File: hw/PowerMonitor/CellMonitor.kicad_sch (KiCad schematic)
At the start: 25 parts, among them Q1 Q_PMOS_GDS, U5 LM358, U6 LM358, U7 LM358, U8 LM393, U9 74LVC1G32

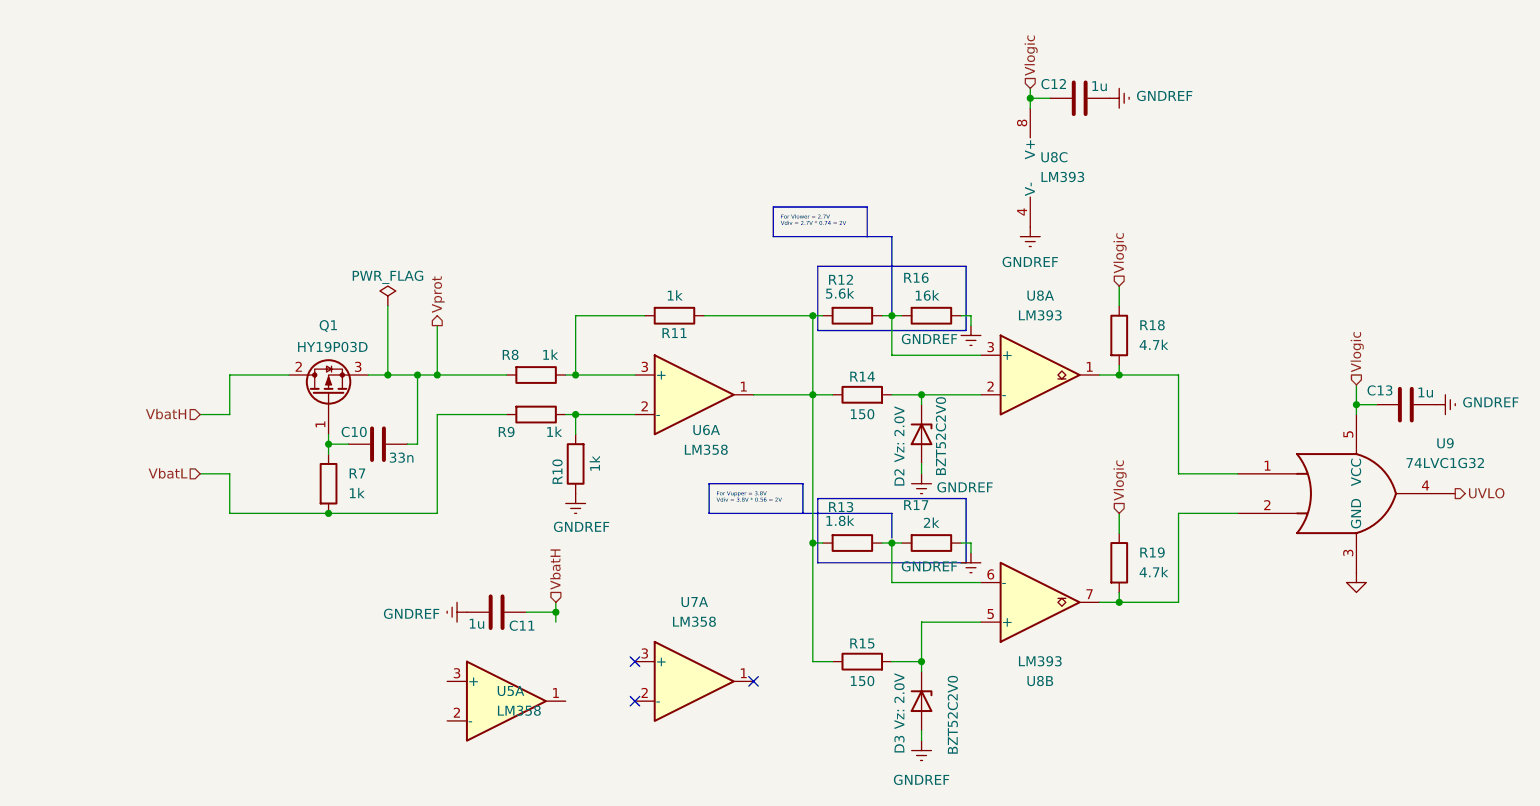
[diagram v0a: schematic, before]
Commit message: Rework powermon
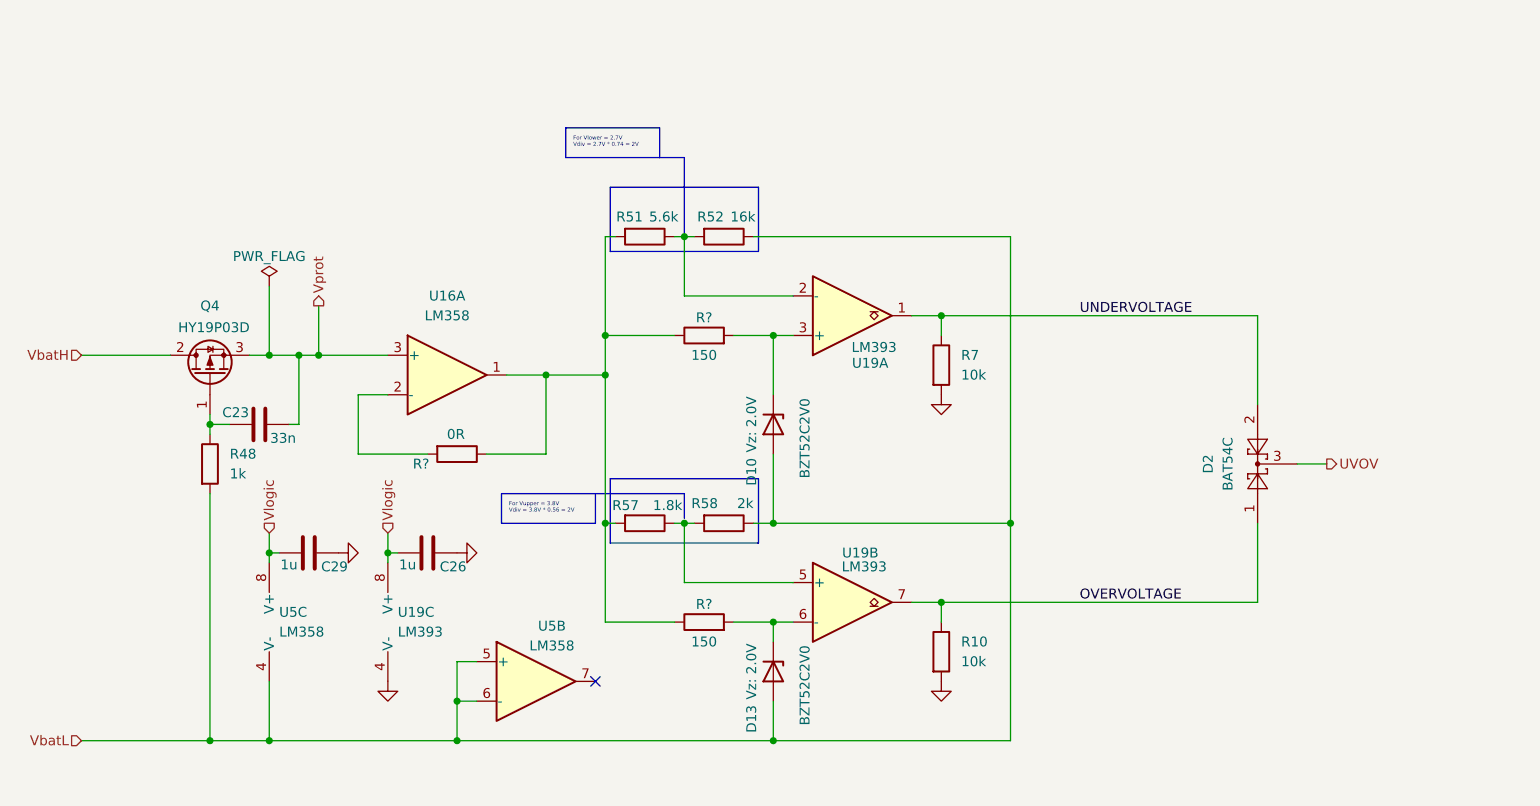
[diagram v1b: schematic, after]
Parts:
- removed C10: 33n, Capacitor_SMD:C_0603_1608Metric_Pad1.08x0.95mm_HandSolder, symbol Device:C
- removed C11, C12, C13: 1u, Capacitor_SMD:C_0603_1608Metric_Pad1.08x0.95mm_HandSolder, symbol Device:C
- removed D2, D3: BZT52Bxx, Diode_SMD:D_SOD-123F, symbol Diode:BZT52Bxx
- removed Q1: Q_PMOS_GDS, Package_TO_SOT_SMD:TO-252-2, symbol Transistor_FET:Q_PMOS_GDS
- removed R11, R8, R9: 1k, Resistor_SMD:R_0603_1608Metric_Pad0.98x0.95mm_HandSolder, symbol Device:R
- removed R12: 5.6k, Resistor_SMD:R_0603_1608Metric_Pad0.98x0.95mm_HandSolder, symbol Device:R
- removed R13: 1.8k, Resistor_SMD:R_0603_1608Metric_Pad0.98x0.95mm_HandSolder, symbol Device:R
- removed R14, R15: 150, Resistor_SMD:R_0603_1608Metric_Pad0.98x0.95mm_HandSolder, symbol Device:R
- removed R16: 16k, Resistor_SMD:R_0603_1608Metric_Pad0.98x0.95mm_HandSolder, symbol Device:R
- removed R17: 2k, Resistor_SMD:R_0603_1608Metric_Pad0.98x0.95mm_HandSolder, symbol Device:R
- removed R18, R19: 4.7k, Resistor_SMD:R_0603_1608Metric_Pad0.98x0.95mm_HandSolder, symbol Device:R
- removed U5, U6, U7: LM358, Package_SO:SOIC-8_3.9x4.9mm_P1.27mm, symbol Amplifier_Operational:LM358
- removed U8: LM393, Package_SO:SOIC-8_3.9x4.9mm_P1.27mm, symbol Comparator:LM393
- removed U9: 74LVC1G32, Package_TO_SOT_SMD:SOT-353_SC-70-5_Handsoldering, symbol 74xGxx:74LVC1G32
- added C23: 33n, Capacitor_SMD:C_0603_1608Metric_Pad1.08x0.95mm_HandSolder, symbol Device:C
- added C26, C29: 1u, Capacitor_SMD:C_0603_1608Metric_Pad1.08x0.95mm_HandSolder, symbol Device:C
- added D10, D13: BZT52Bxx, Diode_SMD:D_SOD-123F, symbol Diode:BZT52Bxx
- added D2: BAT54C, Package_TO_SOT_SMD:SOT-23_Handsoldering, symbol Diode:BAT54C
- added Q4: Q_PMOS_GDS, Package_TO_SOT_SMD:TO-252-2, symbol Transistor_FET:Q_PMOS_GDS
- added R48: 1k, Resistor_SMD:R_0603_1608Metric_Pad0.98x0.95mm_HandSolder, symbol Device:R
- added R51: 5.6k, Resistor_SMD:R_0603_1608Metric_Pad0.98x0.95mm_HandSolder, symbol Device:R
- added R52: 16k, Resistor_SMD:R_0603_1608Metric_Pad0.98x0.95mm_HandSolder, symbol Device:R
- added R57: 1.8k, Resistor_SMD:R_0603_1608Metric_Pad0.98x0.95mm_HandSolder, symbol Device:R
- added R58: 2k, Resistor_SMD:R_0603_1608Metric_Pad0.98x0.95mm_HandSolder, symbol Device:R
- added R?: 0R, Resistor_SMD:R_0603_1608Metric_Pad0.98x0.95mm_HandSolder, symbol Device:R
- added R? (x2): 150, Resistor_SMD:R_0603_1608Metric_Pad0.98x0.95mm_HandSolder, symbol Device:R
- added U16, U5: LM358, Package_SO:SOIC-8_3.9x4.9mm_P1.27mm, symbol Amplifier_Operational:LM358
- added U19: LM393, Package_SO:SOIC-8_3.9x4.9mm_P1.27mm, symbol Comparator:LM393
- R10, R7: value 1k -> 10k
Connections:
- net GND: now also R10.2, R7.2, C26.1, C29.1, U19.4 (V-)
- net VbatH: now also Q4.2 (D)
- net VbatL: now also D10.2 (A), D13.2 (A), R48.2, R52.1, R58.1, U5.4 (V-), U5.5 (+), U5.6 (-); no longer R7.2
- net Vlogic: now also C26.2, C29.2, U19.8 (V+), U5.8 (V+)
- net Vprot: now also C23.2, Q4.3 (S), U16.3 (+)
- net UNDERVOLTAGE: now reaches R7.1
- net UNDERVOLTAGE: now also D2.2, U19.1
- net GNDREF renamed OVERVOLTAGE
- net OVERVOLTAGE: now also D2.1, U19.7
- new net: R51.2, R57.2, R?.1, R?.1, R?.1, U16.1
- new net: R?.2, U16.2 (-)
- new net: R57.1, R58.2, U19.5 (+)
- new net: D13.1 (K), R?.2, U19.6 (-)
- new net: C23.1, Q4.1 (G), R48.1
- new net: R51.1, R52.2, U19.2 (-)
- new net: D10.1 (K), R?.2, U19.3 (+)
- new net UVOV: D2.3
- no-connect marks 3 -> 1
